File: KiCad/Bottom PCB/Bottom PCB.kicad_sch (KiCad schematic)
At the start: 44 parts, among them SW1 SW_MEC_5G, U1 SeeeduinoXIAO

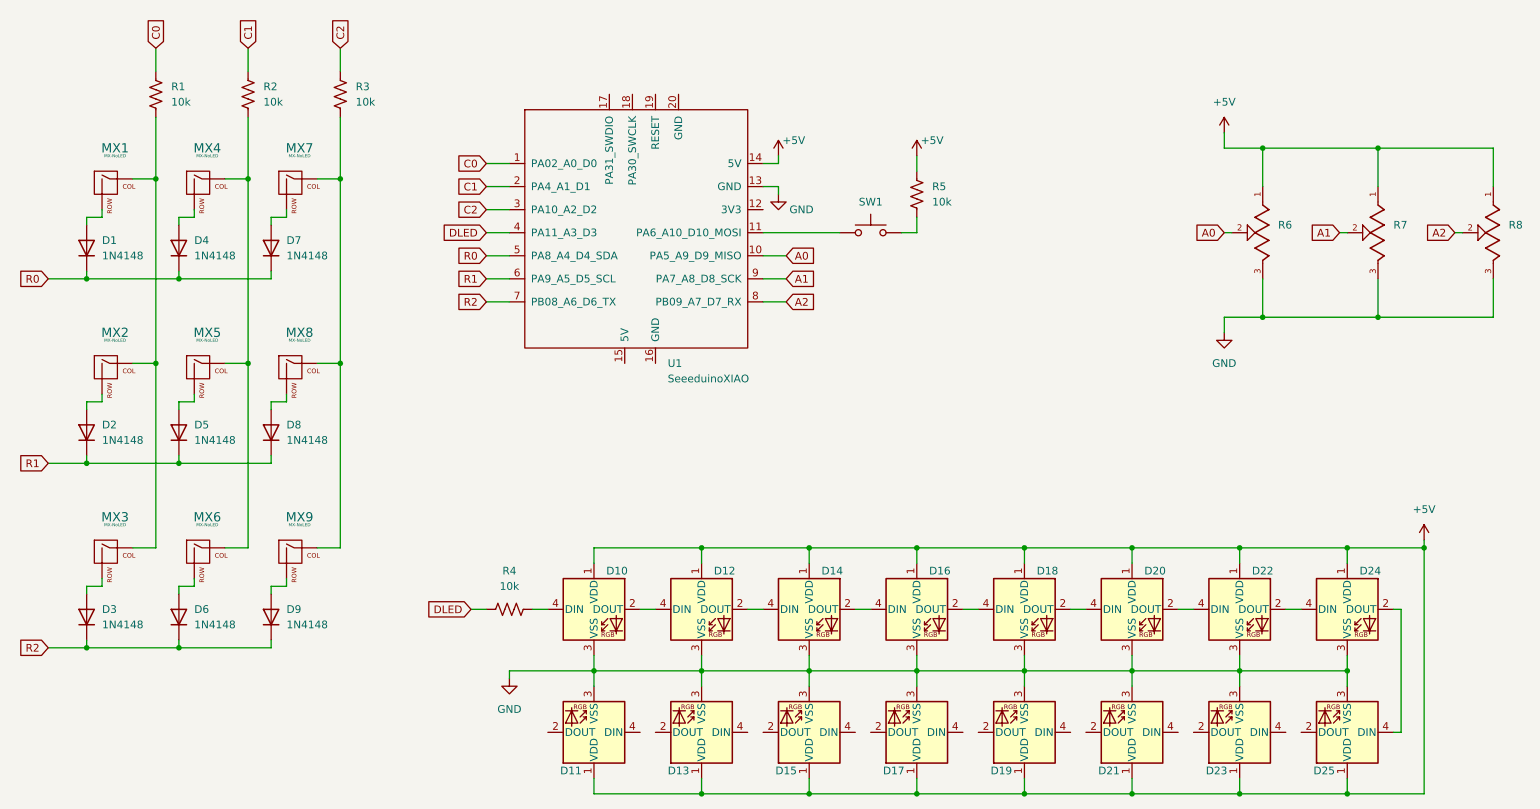
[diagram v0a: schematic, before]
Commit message: Develop bottom PCB
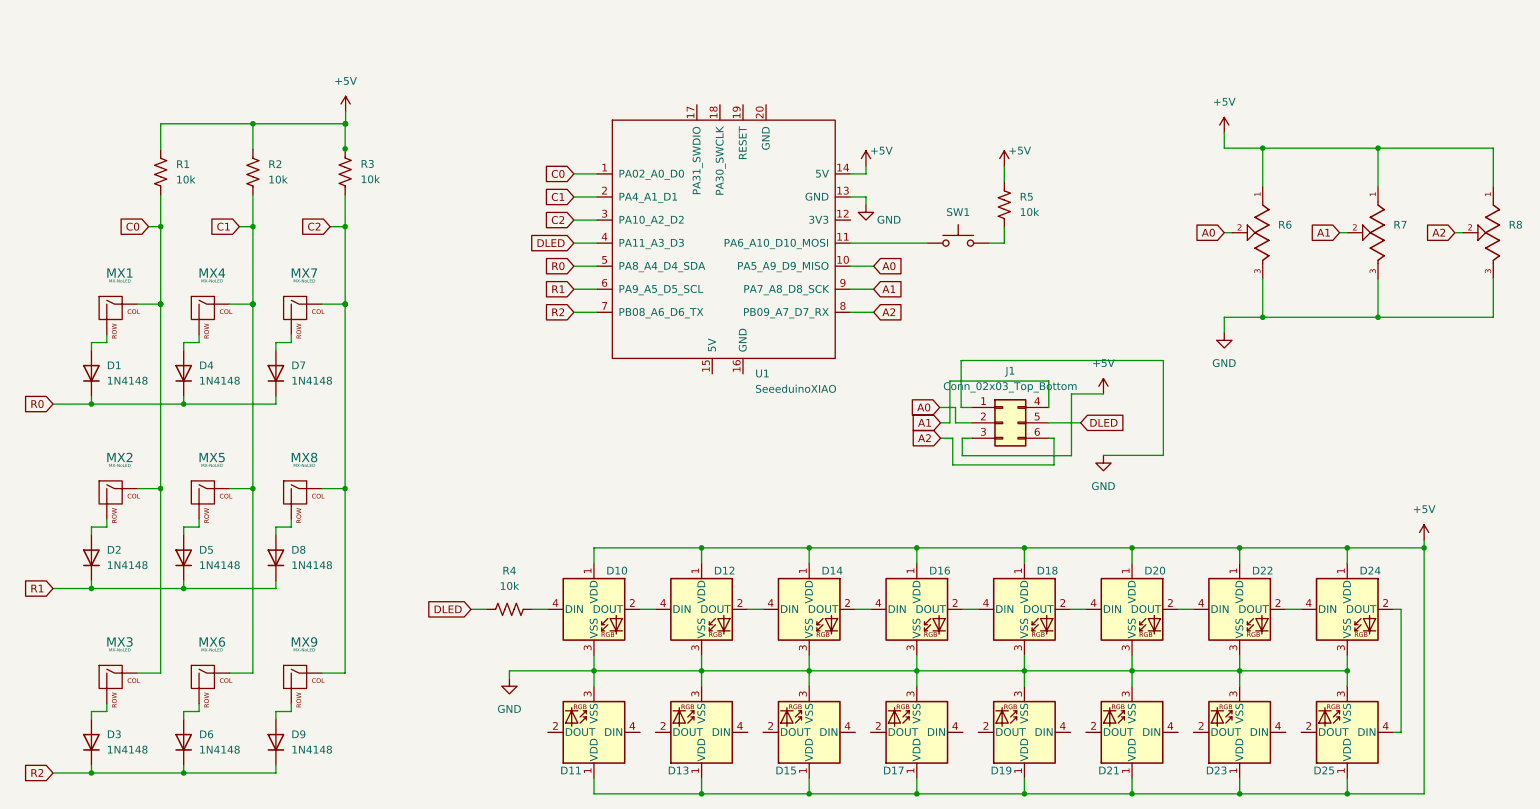
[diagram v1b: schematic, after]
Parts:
- added J1: Conn_02x03_Top_Bottom, Connector_PinHeader_2.54mm:PinHeader_2x03_P2.54mm_Vertical, symbol Connector_Generic:Conn_02x03_Top_Bottom
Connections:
- net +5V: now also R1.1, R2.1, R3.2, J1.3 (Pin_3)
- net A0: now also J1.2 (Pin_2)
- net A1: now also J1.4 (Pin_4)
- net A2: now also J1.6 (Pin_6)
- net C0: now also MX1.1 (COL), MX2.1 (COL), MX3.1 (COL), R1.2; no longer R1.1
- net C1: now also MX4.1 (COL), MX5.1 (COL), MX6.1 (COL), R2.2; no longer R2.1
- net C2: now also MX7.1 (COL), MX8.1 (COL), MX9.1 (COL)
- net DLED: now also J1.5 (Pin_5)
- net GND: now also J1.1 (Pin_1)
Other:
- moved on the sheet: D1, D2, D3, D4, D5, D6, D7, D8, D9, MX1, MX2, MX3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
